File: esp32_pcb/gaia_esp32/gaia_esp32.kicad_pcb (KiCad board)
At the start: 2 copper layers, 101.9 x 70.9 mm, 22 parts, among them J1 supply, J2 motor, J3 Conn_01x03, J4 Switch1, J5 Switch2, J6 Switch3, J7 LED2, J8 LED1, J9 LED3, U1 pcb_power_supply_Vcc_one_supp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, U2 NodeMCU

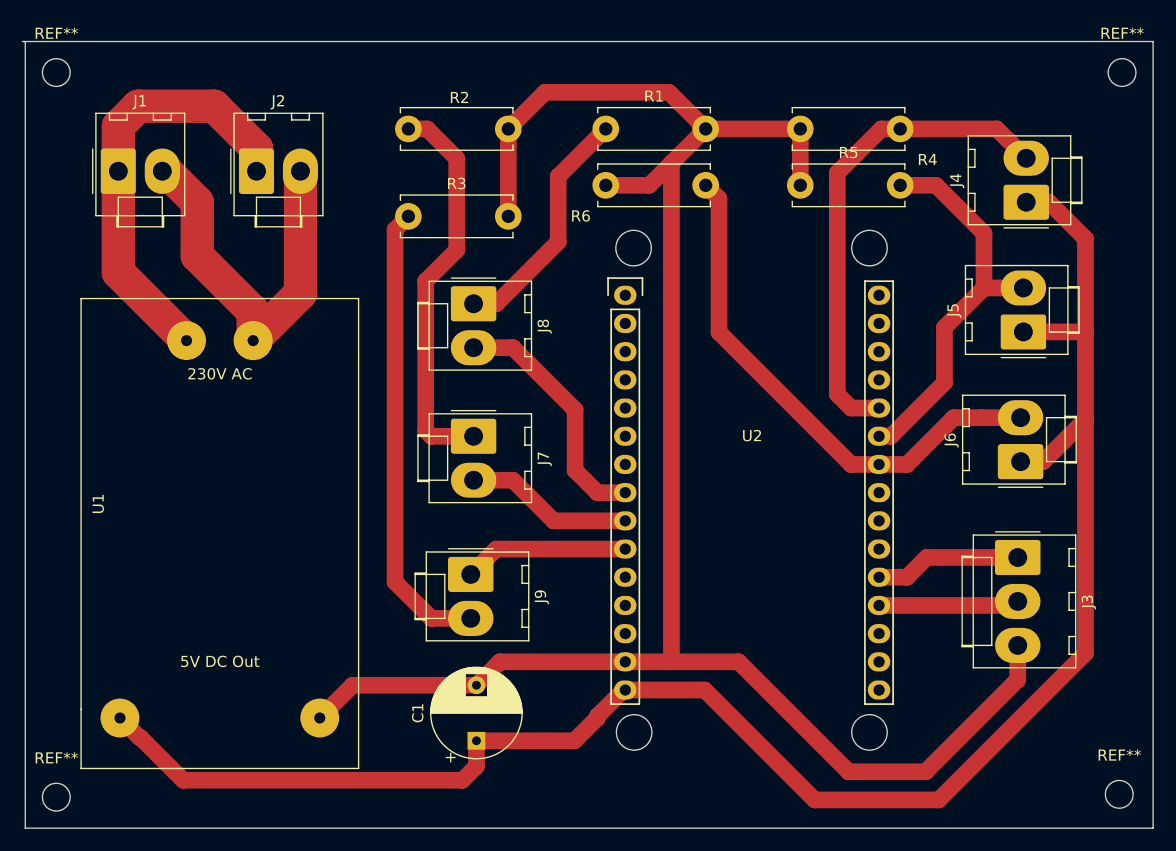
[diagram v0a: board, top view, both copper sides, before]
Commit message: working PCB v2
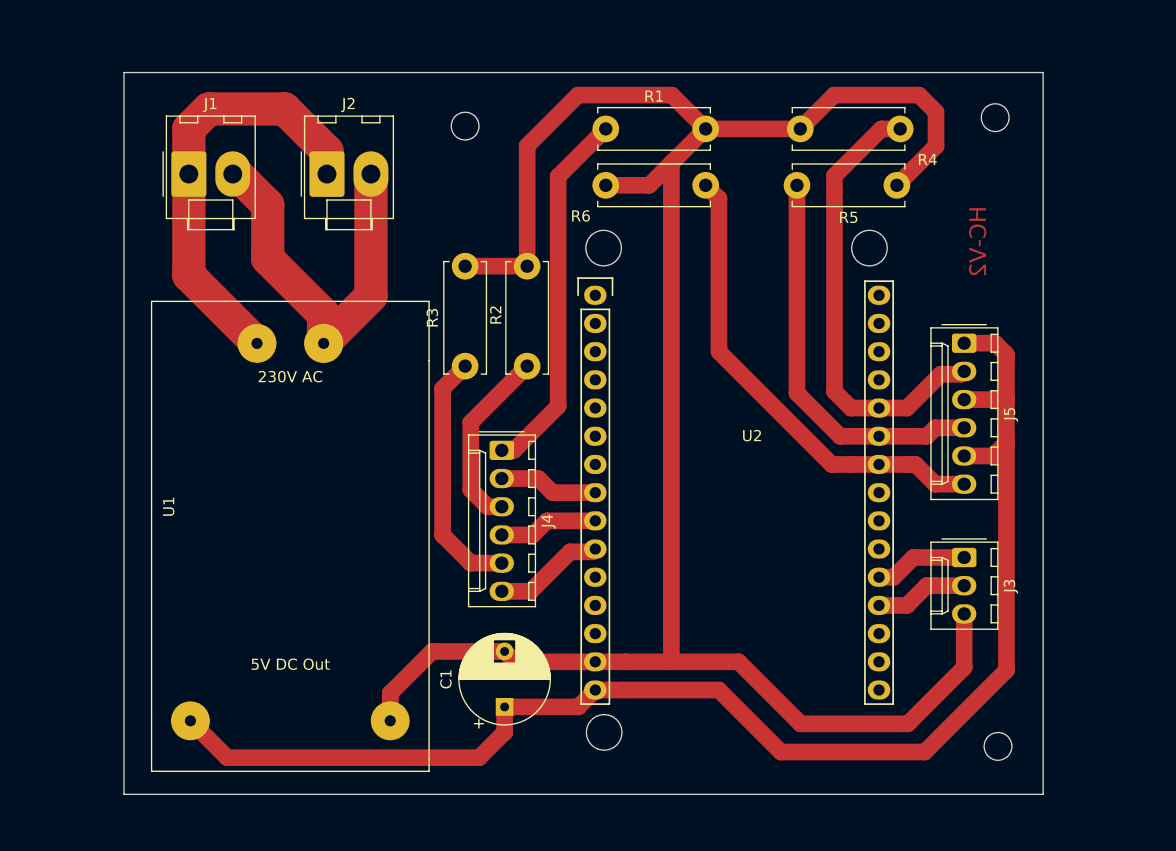
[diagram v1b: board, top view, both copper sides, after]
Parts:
- removed J6: Switch3, Connector_Molex:Molex_KK-396_A-41791-0002_1x02_P3.96mm_Vertical
- removed J7: LED2, Connector_Molex:Molex_KK-396_A-41791-0002_1x02_P3.96mm_Vertical
- removed J8: LED1, Connector_Molex:Molex_KK-396_A-41791-0002_1x02_P3.96mm_Vertical
- removed J9: LED3, Connector_Molex:Molex_KK-396_A-41791-0002_1x02_P3.96mm_Vertical
- removed REF** (x4): MountingHole_2.5mm, MountingHole:MountingHole_2.5mm
- added  : H, MountingHole:MountingHole_2.5mm, F.Cu at (88.1, 40.6)
- added  : H, MountingHole:MountingHole_2.5mm, F.Cu at (136.1, 96.5)
- added  : H, MountingHole:MountingHole_2.5mm, F.Cu at (135.9, 39.9)
- J3: footprint Connector_Molex:Molex_KK-396_A-41791-0003_1x03_P3.96mm_Vertical -> Connector_Molex:Molex_KK-254_AE-6410-03A_1x03_P2.54mm_Vertical
- J4: value Switch1 -> LED_ARRAY; footprint Connector_Molex:Molex_KK-396_A-41791-0002_1x02_P3.96mm_Vertical -> Connector_Molex:Molex_KK-254_AE-6410-06A_1x06_P2.54mm_Vertical
- J5: value Switch2 -> SWITCH_ARRAY; footprint Connector_Molex:Molex_KK-396_A-41791-0002_1x02_P3.96mm_Vertical -> Connector_Molex:Molex_KK-254_AE-6410-06A_1x06_P2.54mm_Vertical
- moved J4 52.3 mm to (91.4, 69.8), turned to 270 degrees
- moved R2 26.6 mm to (93.7, 64.3), turned to 90 degrees
- moved R3 17.0 mm to (88.1, 64.3), turned to 90 degrees
- moved R5 12.7 mm to (129.0, 46.0), turned to 180 degrees
- moved J1 6.36 mm to (63.2, 45.0)
- moved J2 6.36 mm to (75.7, 45.0)
- moved U1 6.36 mm to (72.4, 77.2)
- moved J5 5.43 mm to (133.1, 60.2), turned to 270 degrees
- moved J3 4.83 mm to (133.1, 79.5)
- moved C1 3.97 mm to (91.7, 93.0)
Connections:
- J4 pad 1: +5V -> Net-(J4-Pad1)
- R1 pad 1: Net-(J8-Pad1) -> Net-(J4-Pad1)
- R2 pad 1: Net-(J7-Pad1) -> Net-(J4-Pad3)
- R3 pad 1: Net-(J9-Pad2) -> Net-(J4-Pad5)
- R4 pad 2: Net-(J4-Pad2) -> Net-(J5-Pad2)
- R5 pad 2: Net-(J5-Pad2) -> Net-(J5-Pad4)
- R6 pad 2: Net-(J6-Pad2) -> Net-(J5-Pad6)
- U2 pad 10: Net-(J9-Pad1) -> Net-(J4-Pad6)
- U2 pad 24: Net-(J6-Pad2) -> Net-(J5-Pad6)
- U2 pad 25: Net-(J5-Pad2) -> Net-(J5-Pad4)
- U2 pad 26: Net-(J4-Pad2) -> Net-(J5-Pad2)
- U2 pad 8: Net-(J8-Pad2) -> Net-(J4-Pad2)
- U2 pad 9: Net-(J7-Pad2) -> Net-(J4-Pad4)
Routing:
- net Net-(J6-Pad2): track 47.6 -> 0.00 mm
- net Net-(J5-Pad6): track 0.00 -> 42.5 mm
- net Net-(J9-Pad2): track 41.6 -> 0.00 mm
- net +5V: track 160.7 -> 124.9 mm
- net Net-(J5-Pad4): track 0.00 -> 35.7 mm
- net Net-(J7-Pad1): track 35.7 -> 0.00 mm
- net Net-(J4-Pad2): track 44.0 -> 8.95 mm
- net Net-(J4-Pad1): track 0.00 -> 33.5 mm
- net Net-(J4-Pad5): track 0.00 -> 22.4 mm
- net Net-(J8-Pad2): track 22.3 -> 0.00 mm
- net Net-(J8-Pad1): track 21.9 -> 0.00 mm
- net Net-(J4-Pad3): track 0.00 -> 16.7 mm
- net GND: track 173.6 -> 188.9 mm
- net Net-(J7-Pad2): track 15.2 -> 0.00 mm
- net Net-(J9-Pad1): track 14.9 -> 0.00 mm
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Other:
- board size 101.9 x 70.9 mm -> 82.8 x 65 mm
- board text added: "HC-V2"
